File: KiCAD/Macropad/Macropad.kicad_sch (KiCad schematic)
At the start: 29 parts, among them SW1 SW_Push_45deg, SW2 SW_Push_45deg, SW3 SW_Push_45deg, SW4 SW_Push_45deg, SW5 SW_Push_45deg, SW6 SW_Push_45deg, SW7 EC1110120201, U1 XIAO-RP2040-DIP, U2 SSD1306

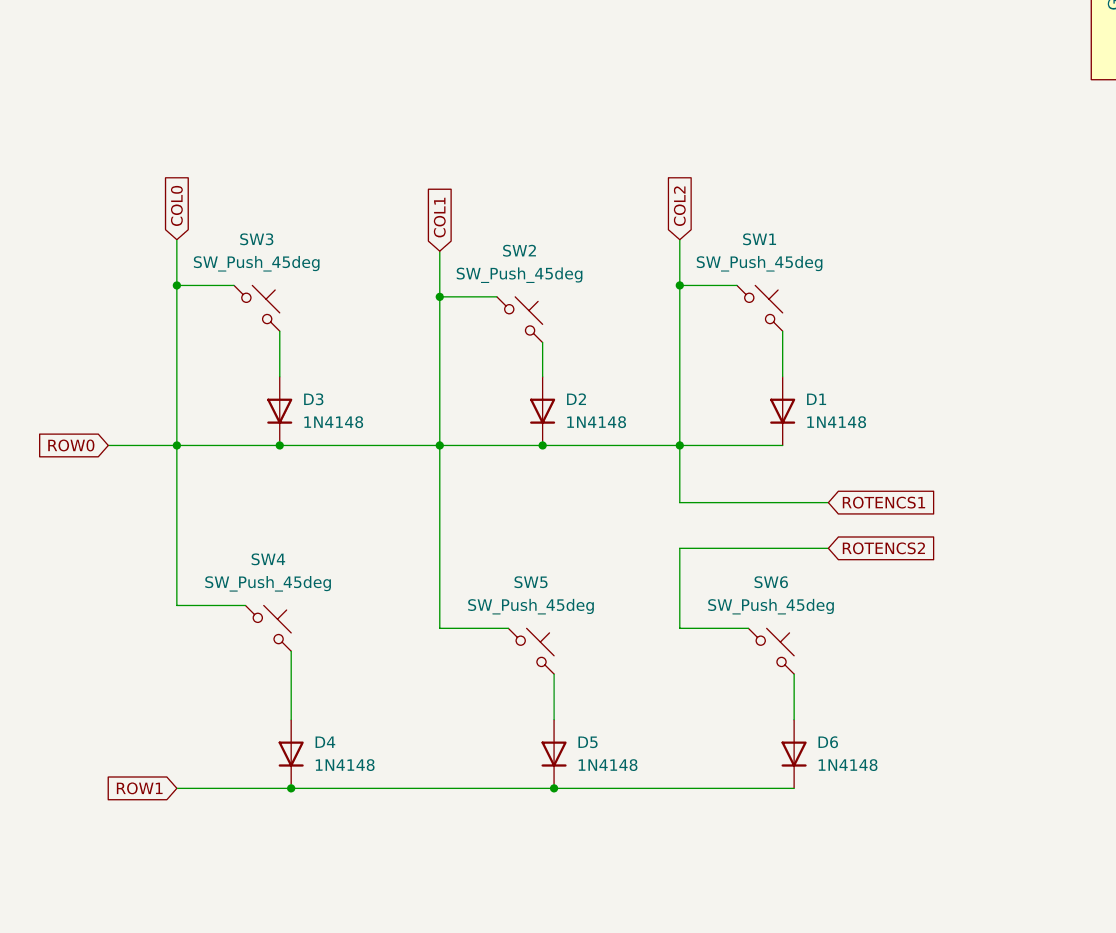
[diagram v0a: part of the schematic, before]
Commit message: Initial candidate for layout
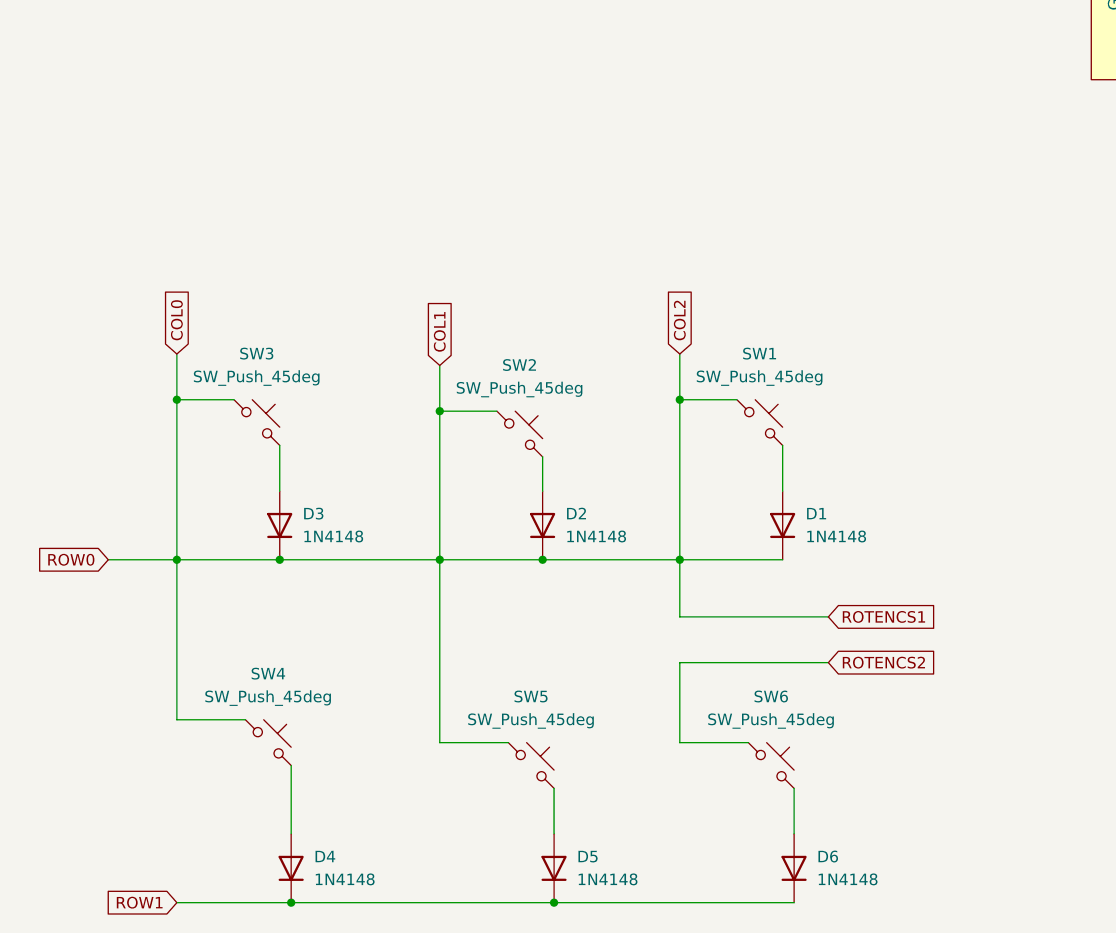
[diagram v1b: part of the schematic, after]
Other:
- moved on the sheet: D1, D2, D3, D4, D5, D6, SW1, SW2, SW3, SW4, SW5, SW6
